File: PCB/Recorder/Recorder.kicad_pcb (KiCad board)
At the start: 2 copper layers, 70 x 70 mm, 50 parts, among them J1 Battery, J2 Reset, J3 TC2030-USB-NL-DS, J4 TF_PUSH, J5 USB-C-Socket-H, Q2 CJ2301, SW2 SW_SPST, U1 R, U2 L, U3 TP4054, U4 ME6211C33M5G-N, U5 NX6020CAKS, U6 ESP32-S3-MINI-1-N4R2

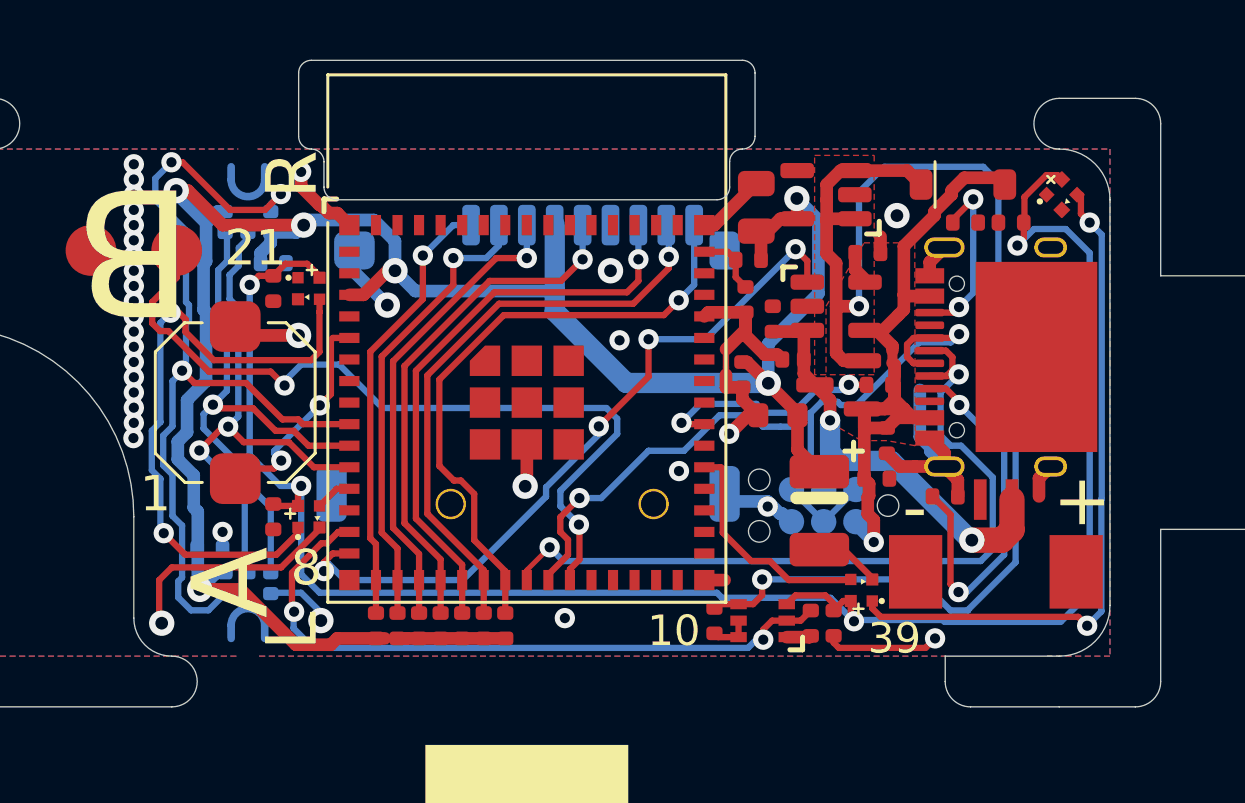
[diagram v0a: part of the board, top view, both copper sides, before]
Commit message: Clean up
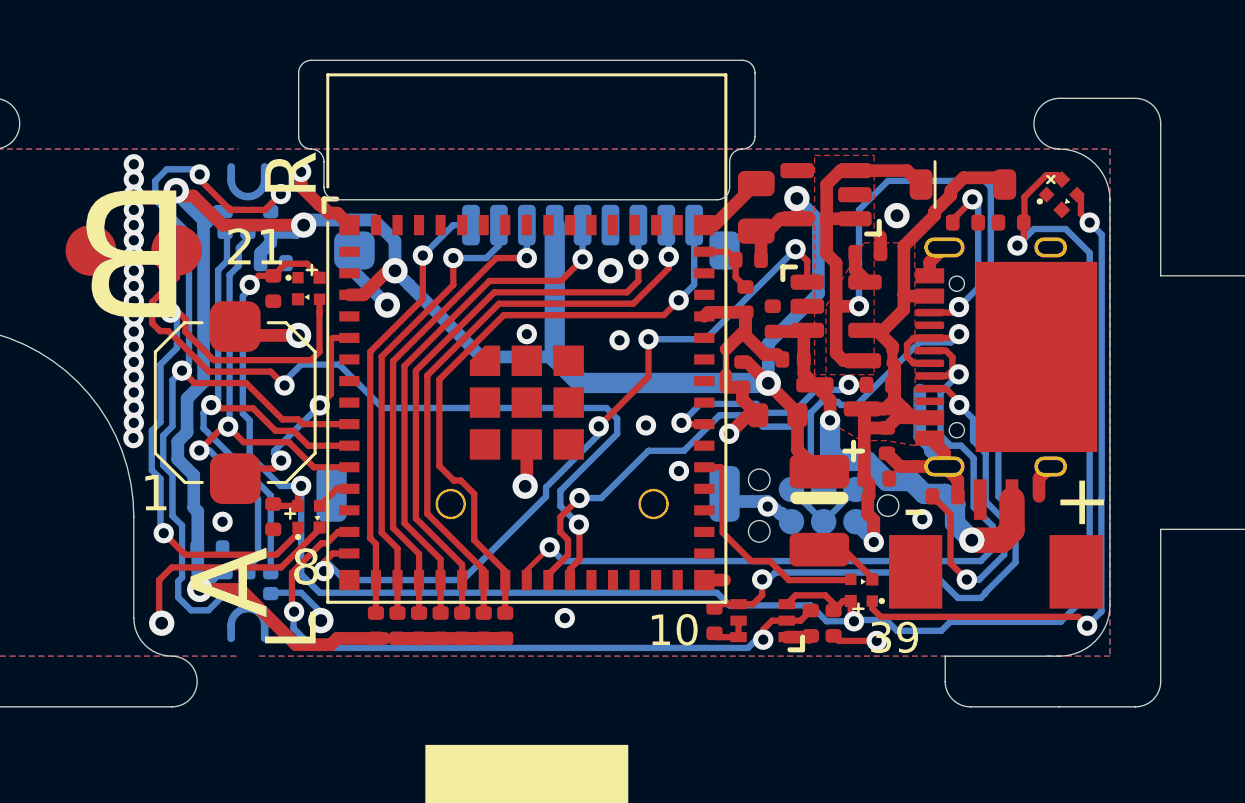
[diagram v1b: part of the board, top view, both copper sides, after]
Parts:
- U4: footprint RevK:SOT-23-5 -> RevK:SOT-23-5-90
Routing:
- net GND: track 60.5 -> 55.7 mm, vias 38 -> 41
- net +3V3: track 84.5 -> 86.5 mm
- net VIN: track 54.1 -> 52.8 mm
- net Net-(J5-CC1): track 14.7 -> 13.9 mm
- net VLED: track 75.3 -> 75.9 mm
- net BUTTON: track 8.68 -> 8.11 mm
